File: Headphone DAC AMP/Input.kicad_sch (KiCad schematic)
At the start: 2 parts, among them J1 USB_C_Receptacle, U2 XU316-1024-QF60B-C24

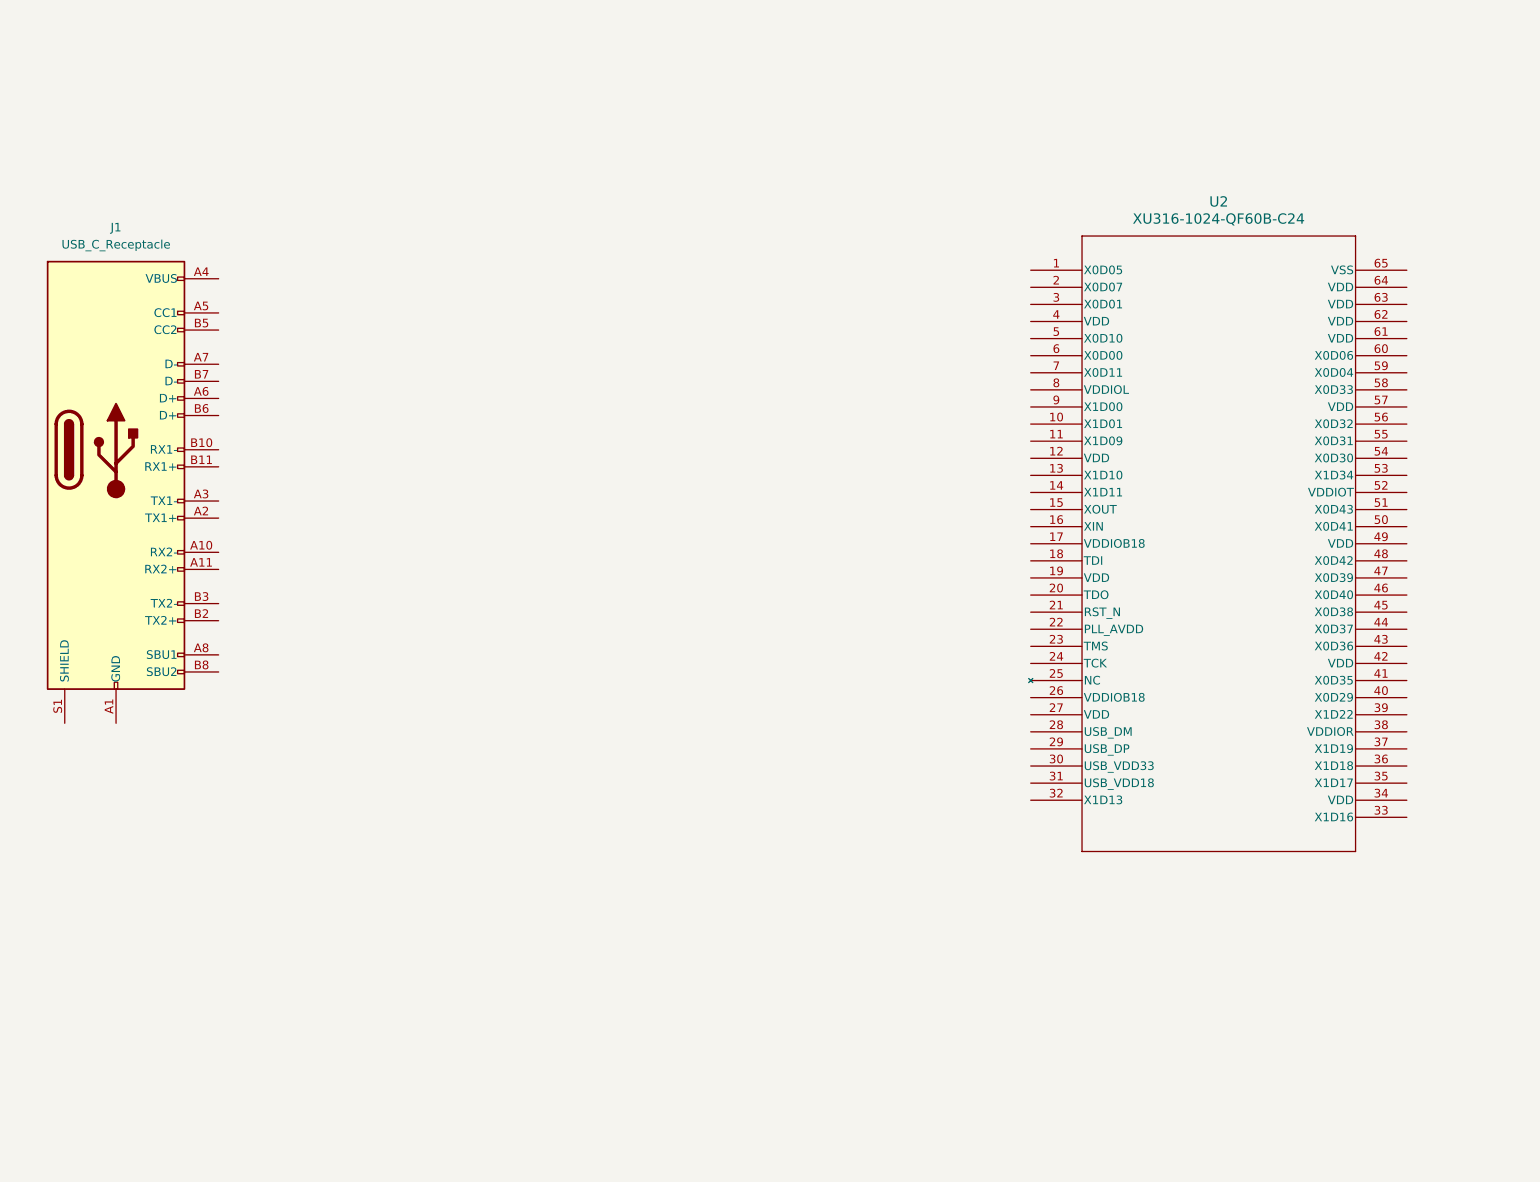
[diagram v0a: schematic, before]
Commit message: Updating Changes
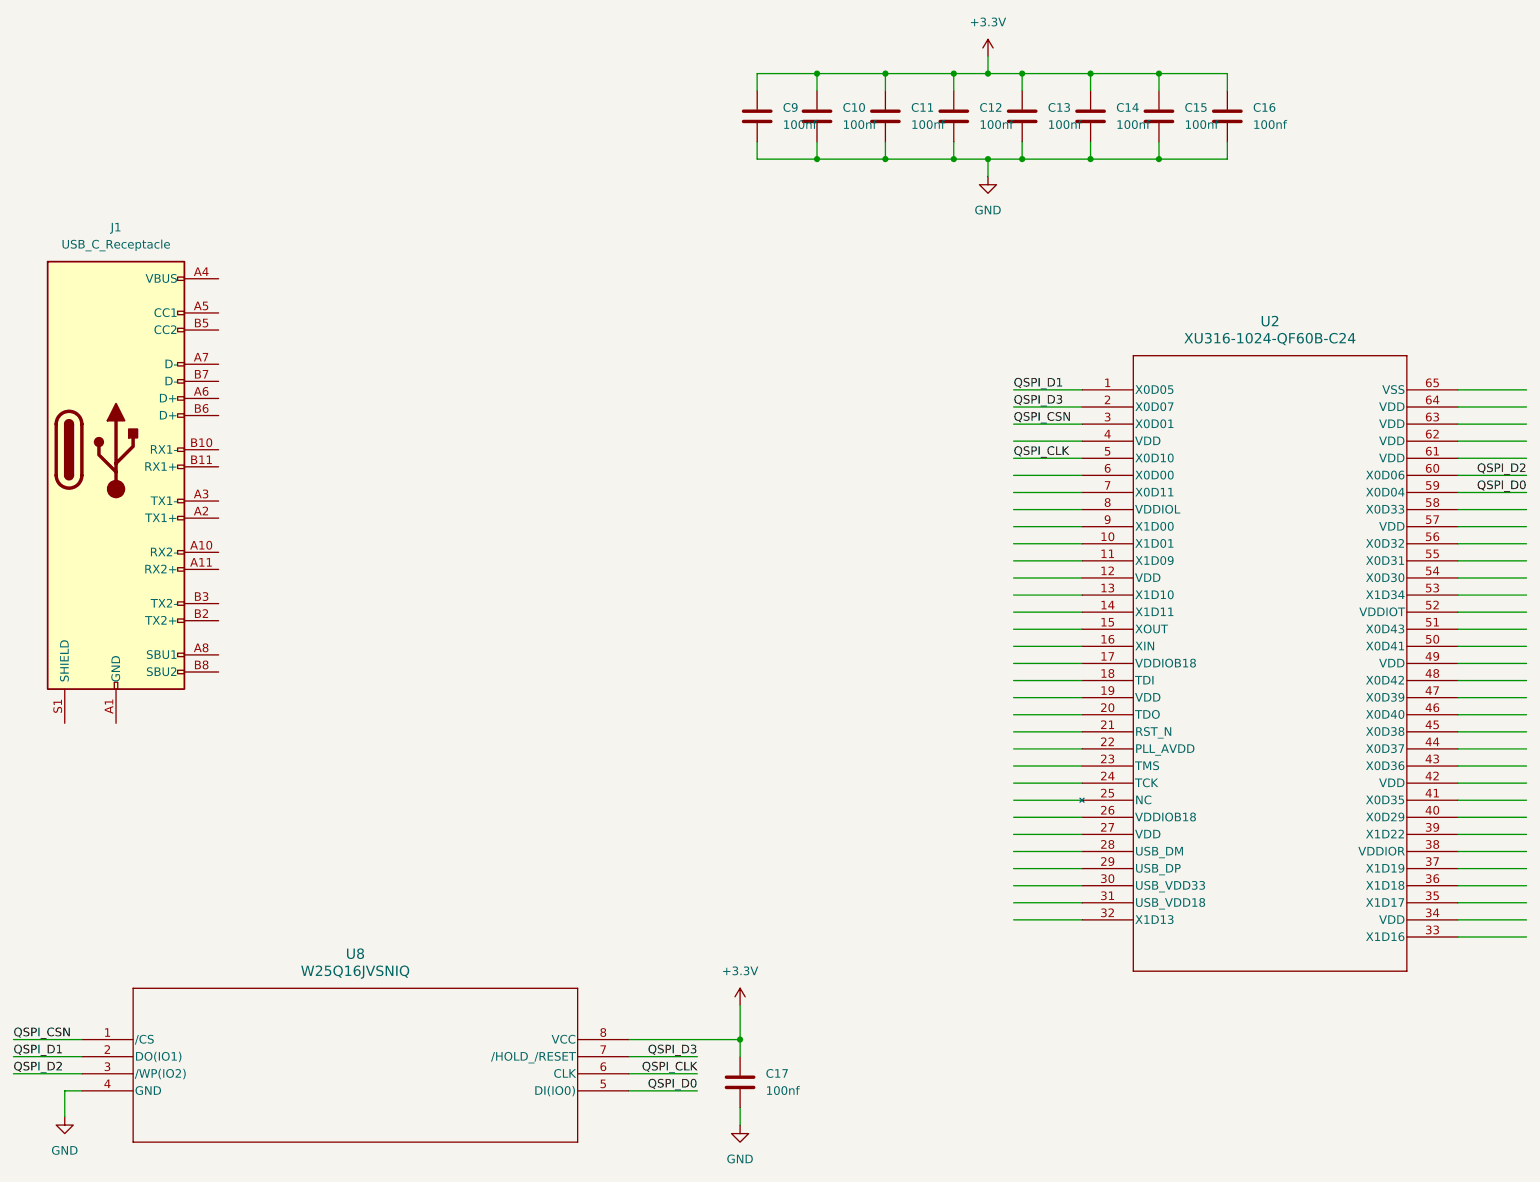
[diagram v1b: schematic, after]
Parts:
- added C10, C11, C12, C13, C14, C15, C16, C17, C9: 100nf, symbol Device:C
- added U8: W25Q16JVSNIQ, SOIC_150MIL_WIN, symbol W25Q16JVSNIQ:W25Q16JVSNIQ
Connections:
- net QSPI_D1: now reaches U2.1 (X0D05)
- net QSPI_D1: now also U8.2 (DO(IO1))
- net QSPI_D3: now reaches U2.2 (X0D07)
- net QSPI_D3: now also U8.7 (/HOLD_/RESET)
- net QSPI_CSN: now reaches U2.3 (X0D01)
- net QSPI_CSN: now also U8.1 (/CS)
- net QSPI_CLK: now reaches U2.5 (X0D10)
- net QSPI_CLK: now also U8.6 (CLK)
- net QSPI_D0: now reaches U2.59 (X0D04)
- net QSPI_D0: now also U8.5 (DI(IO0))
- net QSPI_D2: now reaches U2.60 (X0D06)
- net QSPI_D2: now also U8.3 (/WP(IO2))
- new net +3.3V: C10.1, C11.1, C12.1, C13.1, C14.1, C15.1, C16.1, C17.1, C9.1, U8.8 (VCC)
- new net GND: C10.2, C11.2, C12.2, C13.2, C14.2, C15.2, C16.2, C17.2, C9.2, U8.4 (GND)
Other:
- moved on the sheet: U2
